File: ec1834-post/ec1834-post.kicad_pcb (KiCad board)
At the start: 2 copper layers, 100 x 88 mm, 17 parts, among them U0 BUS_EC1834_8Bit, U1 7432, U2 74HC04, U3 7430, U4 74HC374, U5 2732, U6 2732

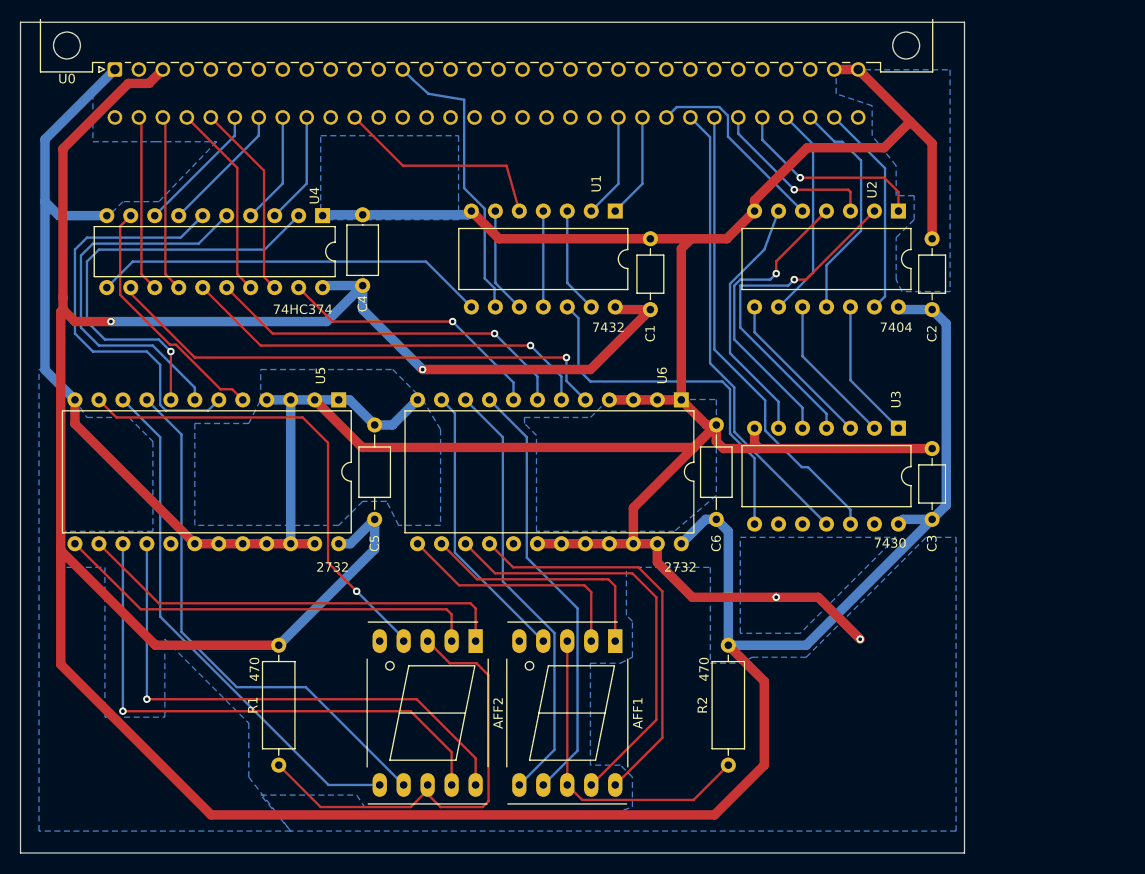
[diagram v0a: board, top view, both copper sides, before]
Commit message: New revision routing still in progress
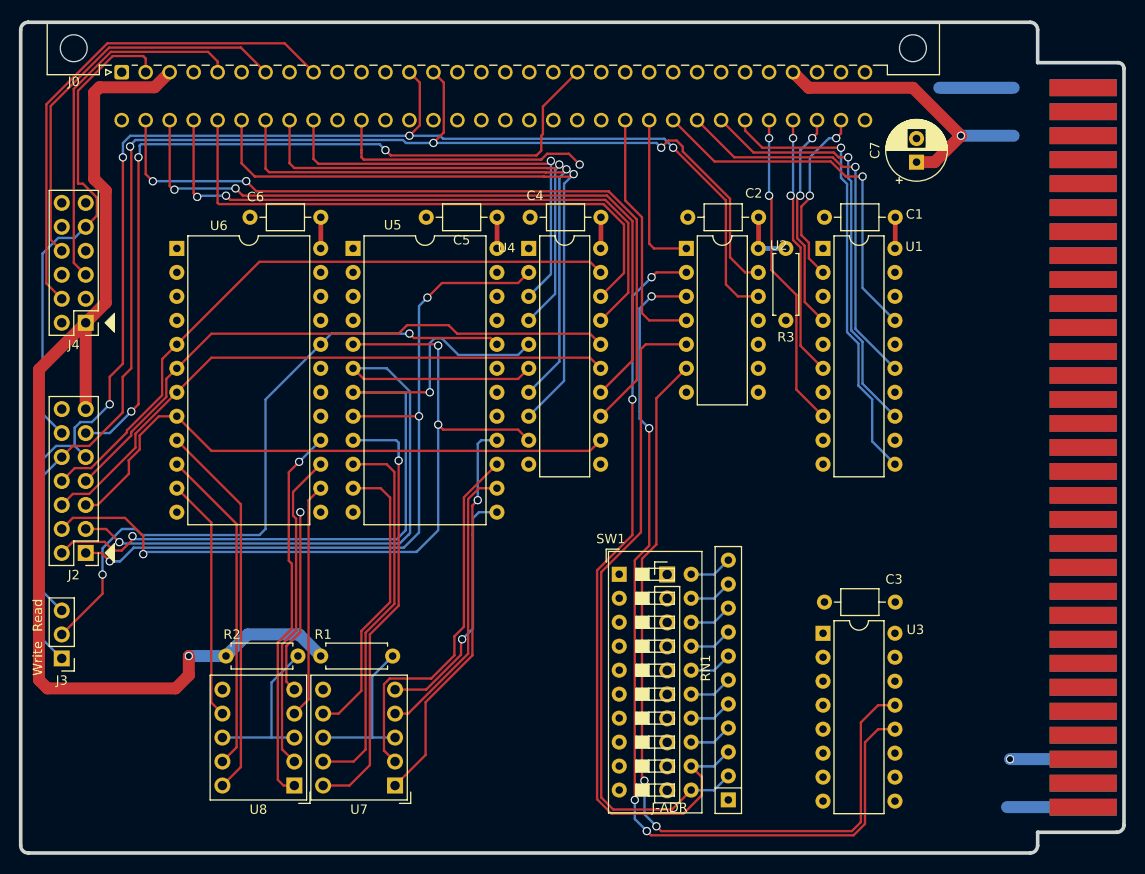
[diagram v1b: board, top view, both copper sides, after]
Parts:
- removed AFF1, AFF2: LTS-6960HR, Display_7Segment:7SegmentLED_LTS6760_LTS6780
- added C7: 100uF 6,3V, Capacitor_THT:CP_Radial_D6.3mm_P2.50mm, F.Cu at (113.9, 35.8)
- added J-ADR: IO-ADDR, Connector_PinHeader_2.54mm:PinHeader_1x10_P2.54mm_Vertical, F.Cu at (87.5, 79.5)
- added J1: Bus_ISA_8bit, Connector_PCBEdge:ISA-8BIT-XT-IDE, F.Cu at (131.8, 66.0)
- added J2: Conn_02x07_Odd_Even, Connector_PinHeader_2.54mm:PinHeader_2x07_P2.54mm_Vertical, F.Cu at (25.9, 77.2)
- added J3: Conn_01x03, Connector_PinHeader_2.54mm:PinHeader_1x03_P2.54mm_Vertical, F.Cu at (23.4, 88.4)
- added J4: Conn_02x06_Odd_Even, Connector_PinHeader_2.54mm:PinHeader_2x06_P2.54mm_Vertical, F.Cu at (25.9, 52.8)
- added R3: 2K2, Resistor_THT:R_Axial_DIN0207_L6.3mm_D2.5mm_P7.62mm_Horizontal, F.Cu at (100.1, 52.6)
- added RN1: R_Network10, Resistor_THT:R_Array_SIP11, F.Cu at (94.0, 103.4)
- added SW1: SW_DIP_x10, Button_Switch_THT:SW_DIP_SPSTx10_Slide_9.78x27.58mm_W7.62mm_P2.54mm, F.Cu at (82.4, 79.5)
- added U7: SA39-11EWA, Display_7Segment:Sx39-1xxxxx, F.Cu at (58.7, 101.9)
- added U8: SA39-11EWA, Display_7Segment:Sx39-1xxxxx, F.Cu at (48.0, 101.9)
- C4: footprint Capacitor_THT:C_Axial_L5.1mm_D3.1mm_P7.50mm_Horizontal -> Capacitor_THT:C_Axial_L3.8mm_D2.6mm_P7.50mm_Horizontal
- C5, C6: footprint Capacitor_THT:C_Axial_L5.1mm_D3.1mm_P10.00mm_Horizontal -> Capacitor_THT:C_Axial_L3.8mm_D2.6mm_P7.50mm_Horizontal
- R1, R2: footprint Resistor_THT:R_Axial_DIN0309_L9.0mm_D3.2mm_P12.70mm_Horizontal -> Resistor_THT:R_Axial_DIN0207_L6.3mm_D2.5mm_P7.62mm_Horizontal
- U1: value 7432 -> 74LS688; footprint Package_DIP:DIP-14_W10.16mm -> Package_DIP:DIP-20_W7.62mm
- U2: value 74HC04 -> 74LS86; footprint Package_DIP:DIP-14_W10.16mm -> Package_DIP:DIP-14_W7.62mm
- U3: value 7430 -> 7432; footprint Package_DIP:DIP-14_W10.16mm -> Package_DIP:DIP-16_W7.62mm
- moved U6 55.8 mm to (35.6, 45.0), turned to 0 degrees
- moved C6 52.7 mm to (50.8, 41.7), turned to 180 degrees
- moved R2 47.0 mm to (48.4, 88.1), turned to 180 degrees
- moved C5 34.5 mm to (69.5, 41.7), turned to 180 degrees
- moved C1 27.7 mm to (111.7, 41.7), turned to 180 degrees
- moved C4 26.3 mm to (80.5, 41.7), turned to 180 degrees
- moved U3 23.1 mm to (104.0, 85.7), turned to 0 degrees
- moved U2 22.8 mm to (89.5, 45.0), turned to 0 degrees
- moved U1 22.4 mm to (104.0, 45.0), turned to 0 degrees
- moved U4 22.1 mm to (72.8, 45.0), turned to 0 degrees
- moved C2 20.8 mm to (97.2, 41.7), turned to 180 degrees
- moved R1 16.7 mm to (58.4, 88.1), turned to 180 degrees
- moved U5 16.1 mm to (54.2, 45.0), turned to 0 degrees
- moved C3 9.59 mm to (111.7, 82.4), turned to 180 degrees
- moved J0 0.77 mm to (29.7, 26.3)
- renumbered U0 to J0
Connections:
- net Net-(U4-Pad2) renamed /DB0
- net Net-(U4-Pad5) renamed /DB1
- net Net-(U4-Pad6) renamed /DB2
- net Net-(U4-Pad9) renamed /DB3
- J0 pad a14: Net-(U0-Pada14) -> IOR
- J0 pad a2: Net-(U0-Pada2) -> RESET
- J0 pad a20: Net-(U0-Pada20) -> CLK
- J0 pad a29: Net-(U0-Pada29) -> +5V
- J0 pad a5: Net-(U0-Pada5) -> -5V
- J0 pad a7: Net-(U0-Pada7) -> -12V
- J0 pad a9: Net-(U0-Pada9) -> +12V
- U1 pad 1: A8 -> AEN
- U1 pad 10: Net-(U1-Pad10) -> GND
- U1 pad 11: Net-(U1-Pad11) -> A4
- U1 pad 12: Net-(U1-Pad12) -> Net-(RN1-Pad7)
- U1 pad 13: Net-(U1-Pad13) -> A5
- U1 pad 14: +5V -> Net-(RN1-Pad6)
- U1 pad 2: A9 -> A0
- U1 pad 3: Net-(U1-Pad13) -> Net-(RN1-Pad11)
- U1 pad 4: Net-(U1-Pad11) -> A1
- U1 pad 5: AEN -> Net-(RN1-Pad10)
- U1 pad 6: Net-(U1-Pad10) -> A2
- U1 pad 7: GND -> Net-(RN1-Pad9)
- U1 pad 8: Net-(U1-Pad8) -> A3
- U1 pad 9: IOW -> Net-(RN1-Pad8)
- U2 pad 1: A3 -> A8
- U2 pad 10: Net-(U2-Pad10) -> Net-(R3-Pad1)
- U2 pad 11: A1 -> ENLATCH
- U2 pad 12: Net-(U2-Pad12) -> IOW
- U2 pad 13: A0 -> IOR
- U2 pad 2: Net-(U2-Pad2) -> /SW_A8
- U2 pad 3: A4 -> /SELA8
- U2 pad 4: Net-(U2-Pad4) -> A9
- U2 pad 5: A7 -> /SW_A9
- U2 pad 6: Net-(U2-Pad6) -> /SELA9
- U2 pad 9: A2 -> Net-(R3-Pad1)
- U3 pad 1: Net-(U2-Pad12) -> Net-(R3-Pad1)
- U3 pad 10: (no net) -> Net-(U3-Pad10)
- U3 pad 11: A6 -> Net-(U3-Pad11)
- U3 pad 12: A5 -> /SELA8
- U3 pad 13: (no net) -> /SELA9
- U3 pad 2: Net-(U2-Pad10) -> Net-(R3-Pad1)
- U3 pad 3: Net-(U2-Pad8) -> Net-(U3-Pad3)
- U3 pad 4: Net-(U2-Pad2) -> Net-(U3-Pad11)
- U3 pad 5: Net-(U2-Pad4) -> /SEL_AD
- U3 pad 6: Net-(U2-Pad6) -> Net-(U3-Pad10)
- U3 pad 8: Net-(U1-Pad12) -> Net-(U3-Pad8)
- U3 pad 9: (no net) -> ENLATCH
- U4 pad 11: Net-(U1-Pad8) -> Net-(U3-Pad8)
- U4 pad 12: Net-(U4-Pad12) -> /DB4
- U4 pad 15: Net-(U4-Pad15) -> /DB5
- U4 pad 16: Net-(U4-Pad16) -> /DB6
- U4 pad 19: Net-(U4-Pad19) -> /DB7
- U5 pad 20: GND -> IOWIOR
- U6 pad 20: GND -> IOWIOR
- U6 pad 5: Net-(U4-Pad12) -> /DB7
- U6 pad 6: Net-(U4-Pad15) -> /DB6
- U6 pad 7: Net-(U4-Pad16) -> /DB5
- U6 pad 8: Net-(U4-Pad19) -> /DB4
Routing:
- net GND: track 361.6 -> 15.9 mm, vias 2 -> 0
- net +5V: track 373.0 -> 178.9 mm, vias 2 -> 3
- net IOR: track 0.00 -> 141.0 mm, vias 0 -> 3
- net IOW: track 30.9 -> 150.7 mm, vias 0 -> 4
- net /SELA8: track 0.00 -> 98.6 mm, vias 0 -> 4
- net /SELA9: track 0.00 -> 88.3 mm, vias 0 -> 2
- net CLK: track 0.00 -> 87.7 mm, vias 0 -> 3
- net /SW_A8: track 0.00 -> 82.2 mm, vias 0 -> 2
- net IOWIOR: track 0.00 -> 71.4 mm, vias 0 -> 2
- net /SW_A9: track 0.00 -> 69.7 mm
- net /DB7: track 0.00 -> 69.5 mm
- net /DB5: track 0.00 -> 64.9 mm
- net D7: track 18.7 -> 82.6 mm, vias 0 -> 2
- net /DB6: track 0.00 -> 63.6 mm
- net /DB4: track 0.00 -> 62.1 mm
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- removed copper zone on B.Cu, net GND
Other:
- board size 100 x 88 mm -> 116.9 x 88 mm
- net class Default: clearance 0.2 -> 0.19; via_dia 0.8 -> 0.889; via_drill 0.4 -> 0.635
- rule trace_clearance: 0.2 -> 0.19
- rule via_min_drill: 0.3 -> 0.508
- rule via_min_size: 0.4 -> 0.889
- board text added: "Read"
- board text added: "Write"
- board text removed: "2732"
- board text removed: "470"
- board text removed: "7404"
- board text removed: "7430"
- board text removed: "7432"
- board text removed: "74HC374"
